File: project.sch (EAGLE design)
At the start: 44 parts, among them Y1 ABM8-20.000MHZ-B2-T

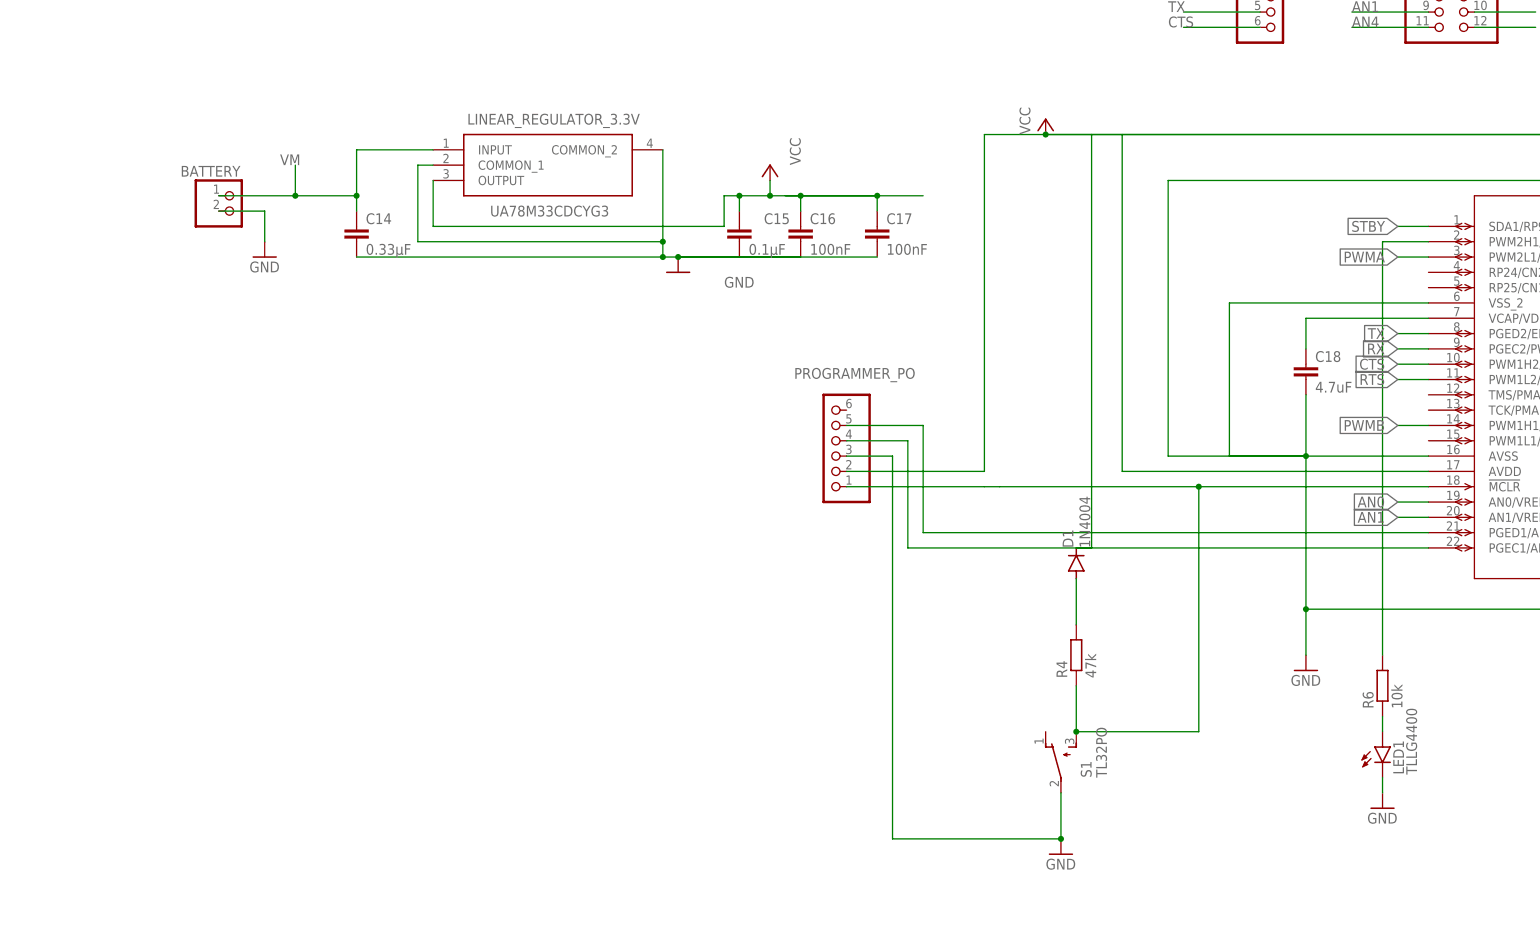
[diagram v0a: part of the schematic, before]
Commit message: Kleine Änderungen
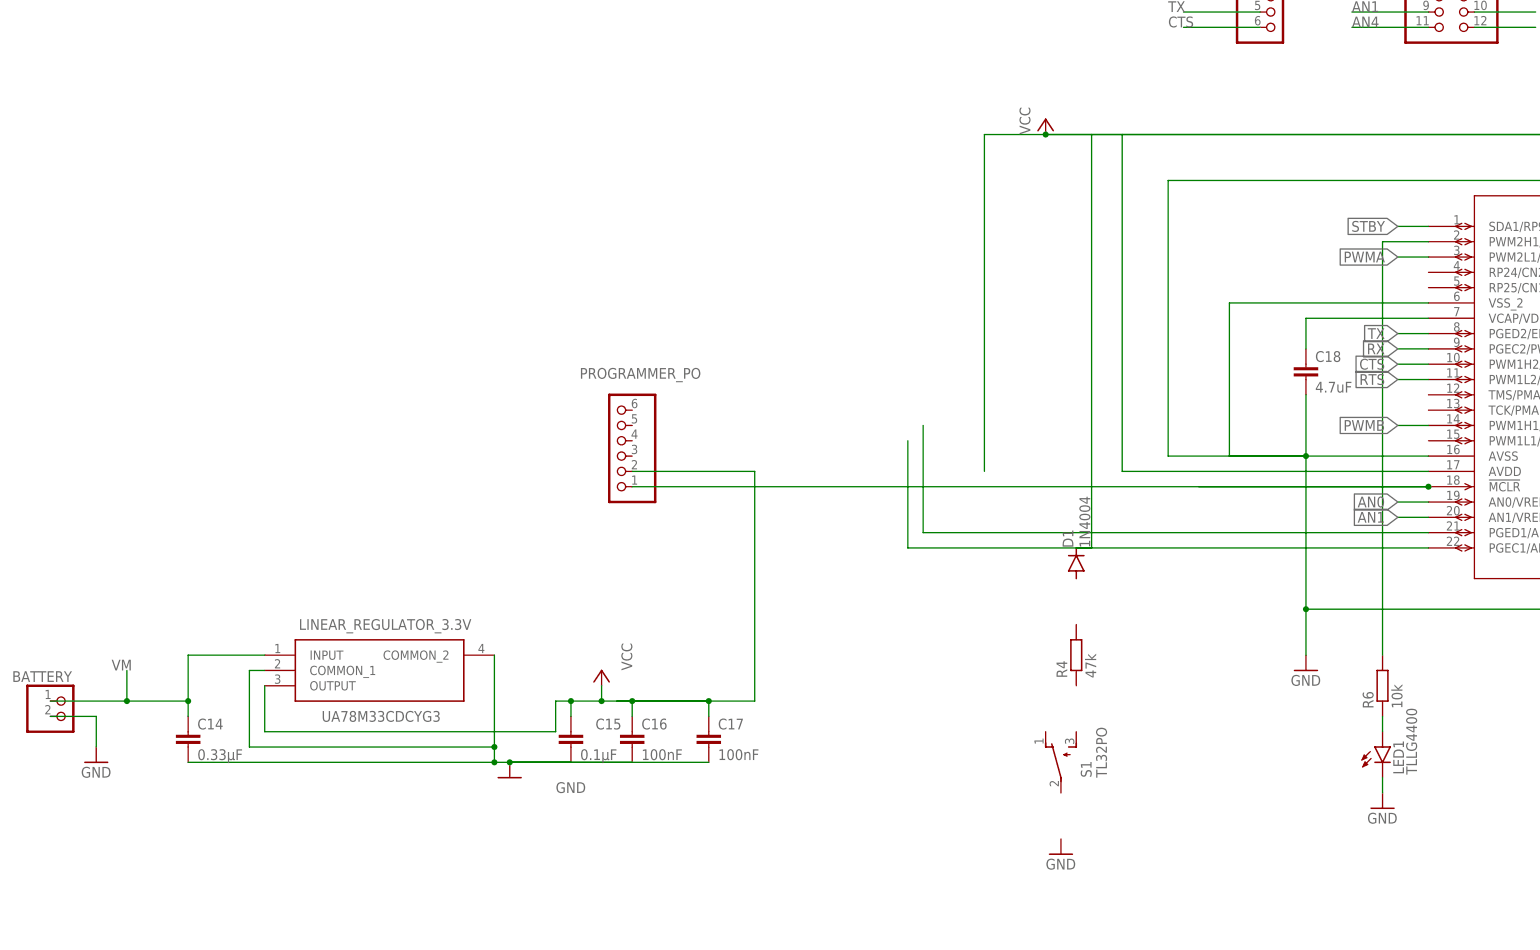
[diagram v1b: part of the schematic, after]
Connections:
- removed net N$9: D1.A, R4.2
- net GND: no longer PROGRAMMER_PO.3, S1.P
- net N$12: no longer PROGRAMMER_PO.4
- net N$13: no longer PROGRAMMER_PO.5
- net N$8: no longer R4.1, S1.S
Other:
- moved on the sheet: BATTERY, C14, C15, C16, C17, LINEAR_REGULATOR_3.3V, PROGRAMMER_PO
